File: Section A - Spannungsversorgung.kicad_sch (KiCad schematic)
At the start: 3 parts, among them Q1 BF459

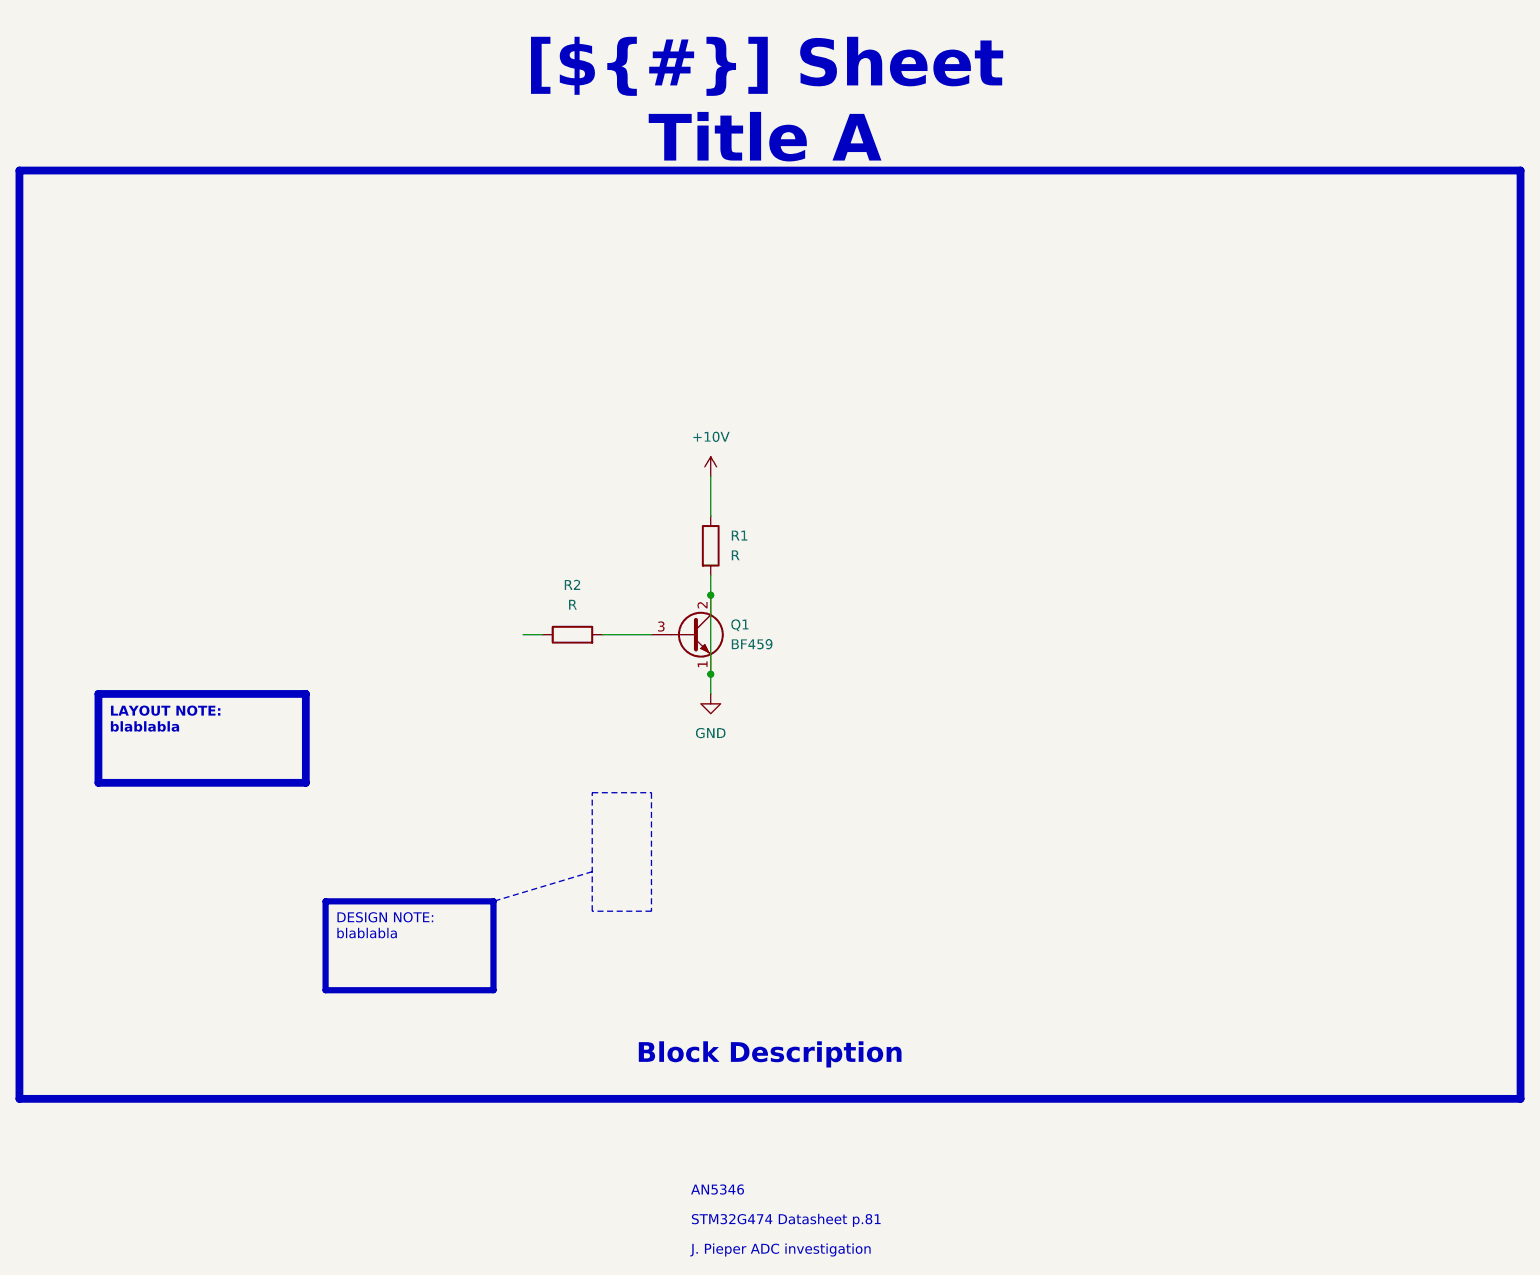
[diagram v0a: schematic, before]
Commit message: nochmal git add .
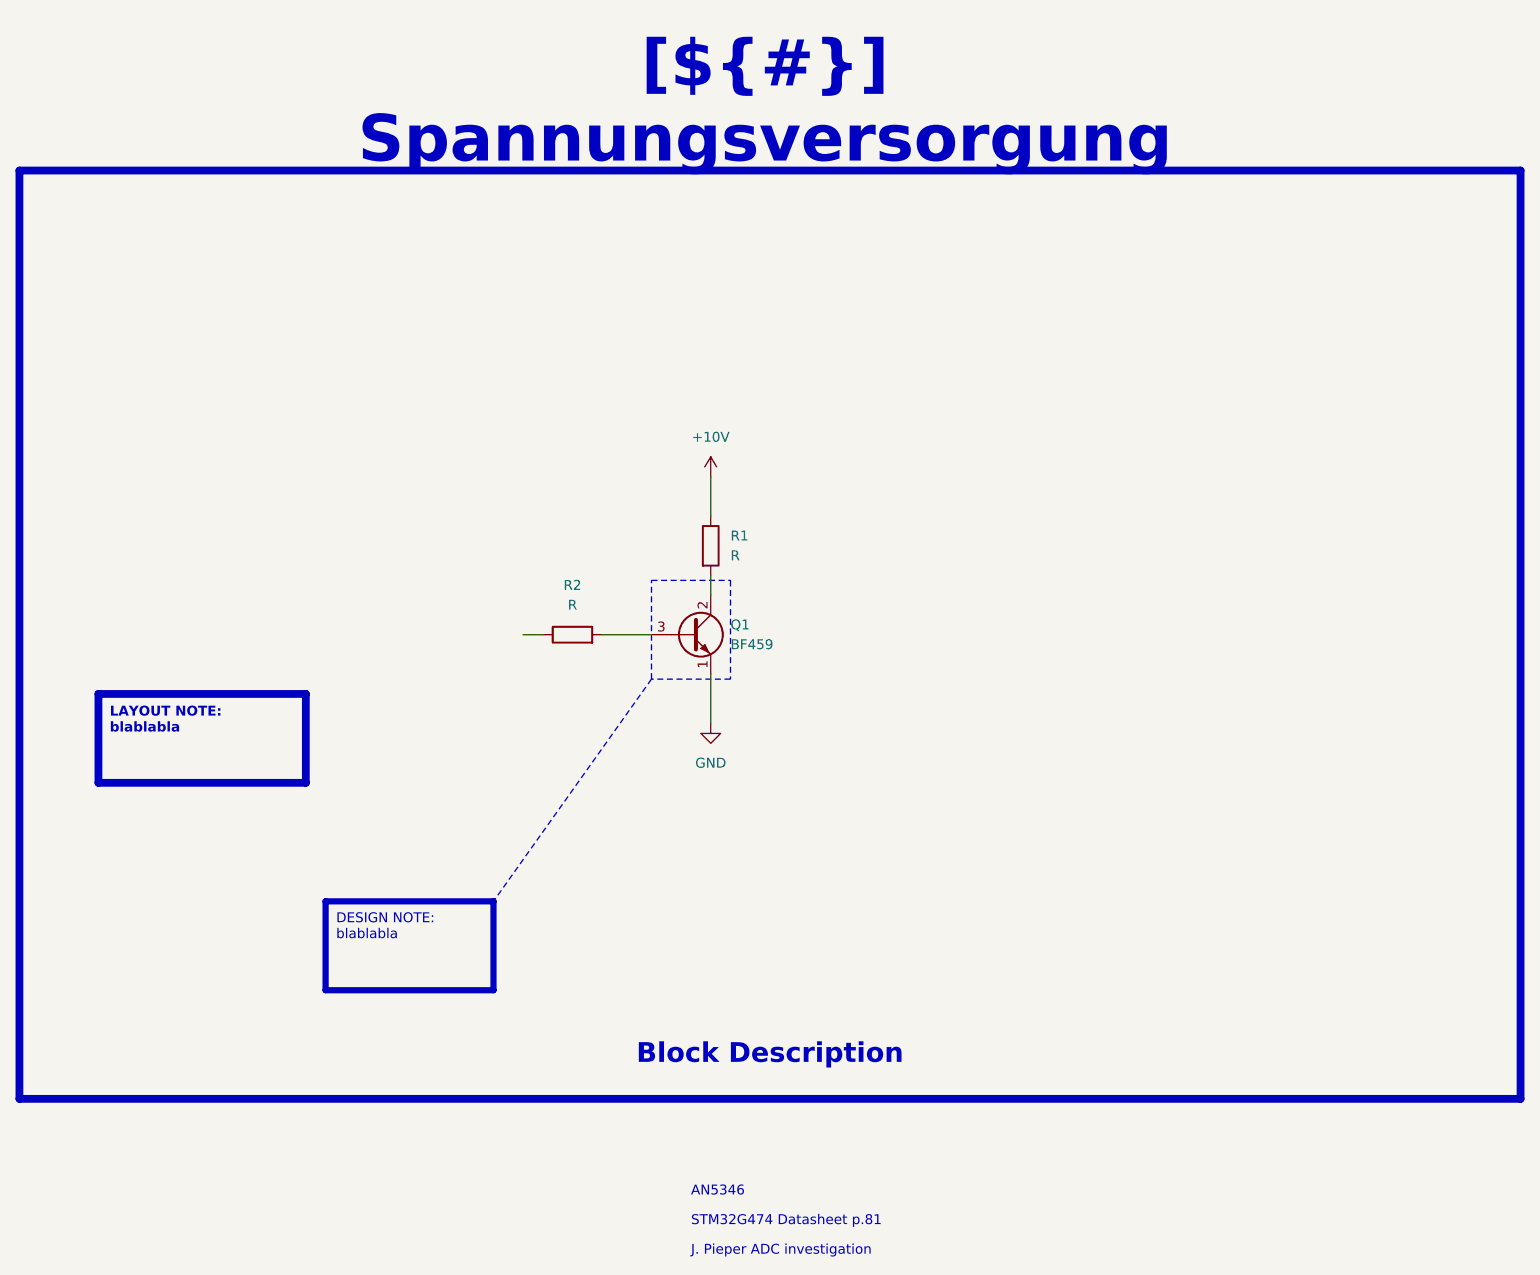
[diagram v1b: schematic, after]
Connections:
- net GND: no longer Q1.2 (C), R1.2
- new net: Q1.2 (C), R1.2
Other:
- title: Sheet Title A -> Spannungsversorgung
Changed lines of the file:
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@@
 	(paper "A4")
 	(title_block
-		(title "Sheet Title A")
+		(title "Spannungsversorgung")
 		(date "2025-01-12")
 		(rev "${REVISION}")
@@
 	)
 	(rectangle
-		(start 129.54 110.49)
-		(end 137.16 125.73)
+		(start 137.16 83.185)
+		(end 147.32 95.885)
 		(stroke
 			(width 0)
@@
 		(stroke
 			(width -0.0001)
-			(type default)
+			(type solid)
 		)
 		(fill
@@
 		(stroke
 			(width -0.0001)
-			(type default)
+			(type solid)
 		)
 		(fill
@@
 		)
 	)
-	(junction
-		(at 144.78 95.25)
-		(diameter 0)
-		(color 0 0 0 0)
-	)
-	(junction
-		(at 144.78 85.09)
-		(diameter 0)
-		(color 0 0 0 0)
-	)
 	(wire
 		(pts
@@
 	(wire
 		(pts
-			(xy 144.78 82.55) (xy 144.78 85.09)
+			(xy 144.78 95.25) (xy 144.78 101.6)
 		)
 		(stroke
@@
 	(wire
 		(pts
-			(xy 144.78 95.25) (xy 144.78 97.79)
+			(xy 144.78 82.55) (xy 144.78 85.09)
 		)
 		(stroke
@@
 	(polyline
 		(pts
-			(xy 129.54 120.65) (xy 116.84 124.46)
+			(xy 137.16 95.885) (xy 116.84 124.46)
 		)
 		(stroke
@@
 			(type dot)
 			(color 255 0 0 1)
-		)
-	)
-	(wire
-		(pts
-			(xy 144.78 85.09) (xy 144.78 95.25)
-		)
-		(stroke
-			(width 0)
-			(type default)
 		)
 	)
@@
 		)
 		(instances
-			(project ""
+			(project "Project Architecture"
 				(path "/07236397-3ba4-47af-9809-3faac3a2aa49/f06537ee-772d-44d3-8c50-e0ba41038c9c"
 					(reference "R1")
@@
 	(symbol
 		(lib_id "power:GND")
-		(at 144.78 97.79 0)
+		(at 144.78 101.6 0)
 		(unit 1)
 		(exclude_from_sim no)
@@
 		(fields_autoplaced yes)
 		(property "Reference" "#PWR01"
-			(at 144.78 104.14 0)
+			(at 144.78 107.95 0)
 			(effects
 				(font
@@
 		)
 		(property "Value" "GND"
-			(at 144.78 102.87 0)
+			(at 144.78 106.68 0)
 			(effects
 				(font
@@
 		)
 		(property "Footprint" ""
-			(at 144.78 97.79 0)
+			(at 144.78 101.6 0)
 			(effects
 				(font
@@
 		)
 		(property "Datasheet" ""
-			(at 144.78 97.79 0)
+			(at 144.78 101.6 0)
 			(effects
 				(font
@@
 		)
 		(property "Description" "Power symbol creates a global label with name \"GND\" , ground"
-			(at 144.78 97.79 0)
+			(at 144.78 101.6 0)
 			(effects
 				(font
@@
 		)
 		(instances
-			(project ""
+			(project "Project Architecture"
 				(path "/07236397-3ba4-47af-9809-3faac3a2aa49/f06537ee-772d-44d3-8c50-e0ba41038c9c"
 					(reference "#PWR01")
@@
 		)
 		(instances
-			(project ""
+			(project "Project Architecture"
 				(path "/07236397-3ba4-47af-9809-3faac3a2aa49/f06537ee-772d-44d3-8c50-e0ba41038c9c"
 					(reference "Q1")
@@
 		)
 		(instances
-			(project ""
+			(project "Project Architecture"
 				(path "/07236397-3ba4-47af-9809-3faac3a2aa49/f06537ee-772d-44d3-8c50-e0ba41038c9c"
 					(reference "#PWR02")
